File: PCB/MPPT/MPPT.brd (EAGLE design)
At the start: 2 parts, among them IC1 ACS711KEXLT-15AB-T, IC2 ACS711KEXLT-15AB-T

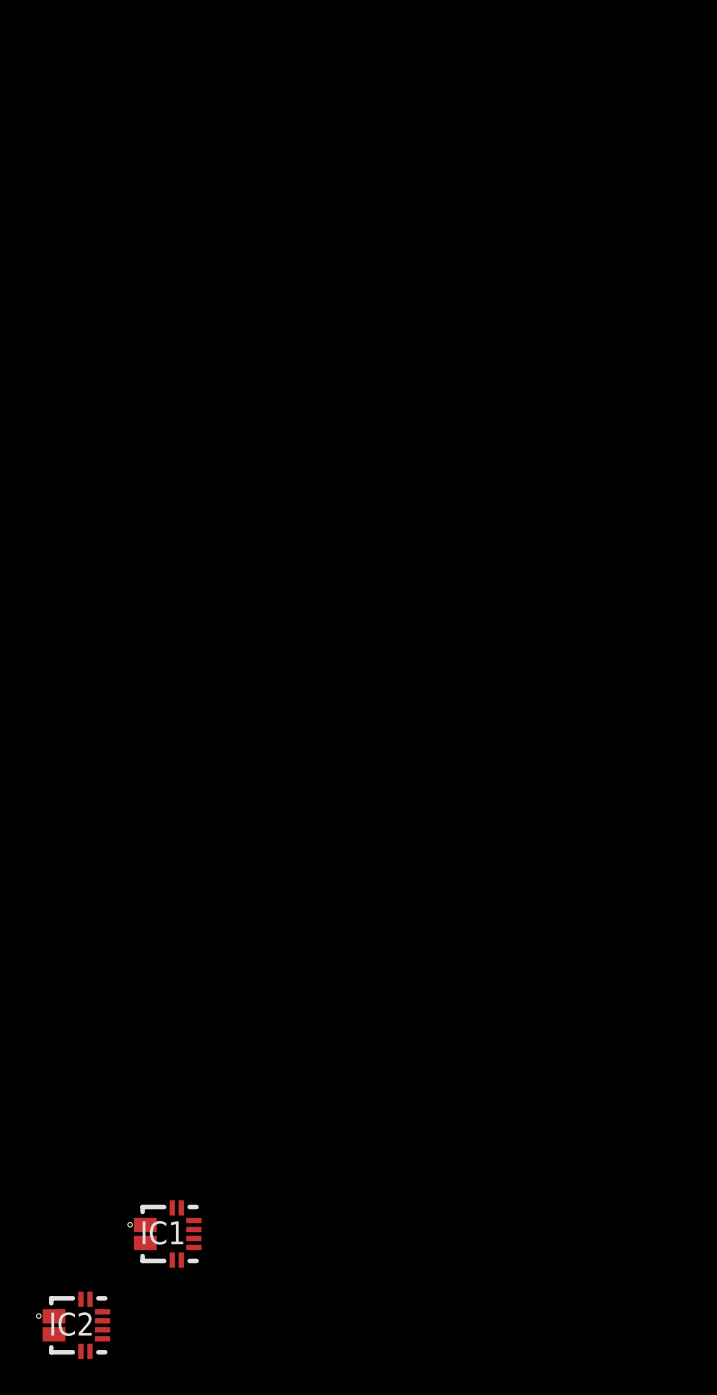
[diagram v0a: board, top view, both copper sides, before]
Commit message: ripup
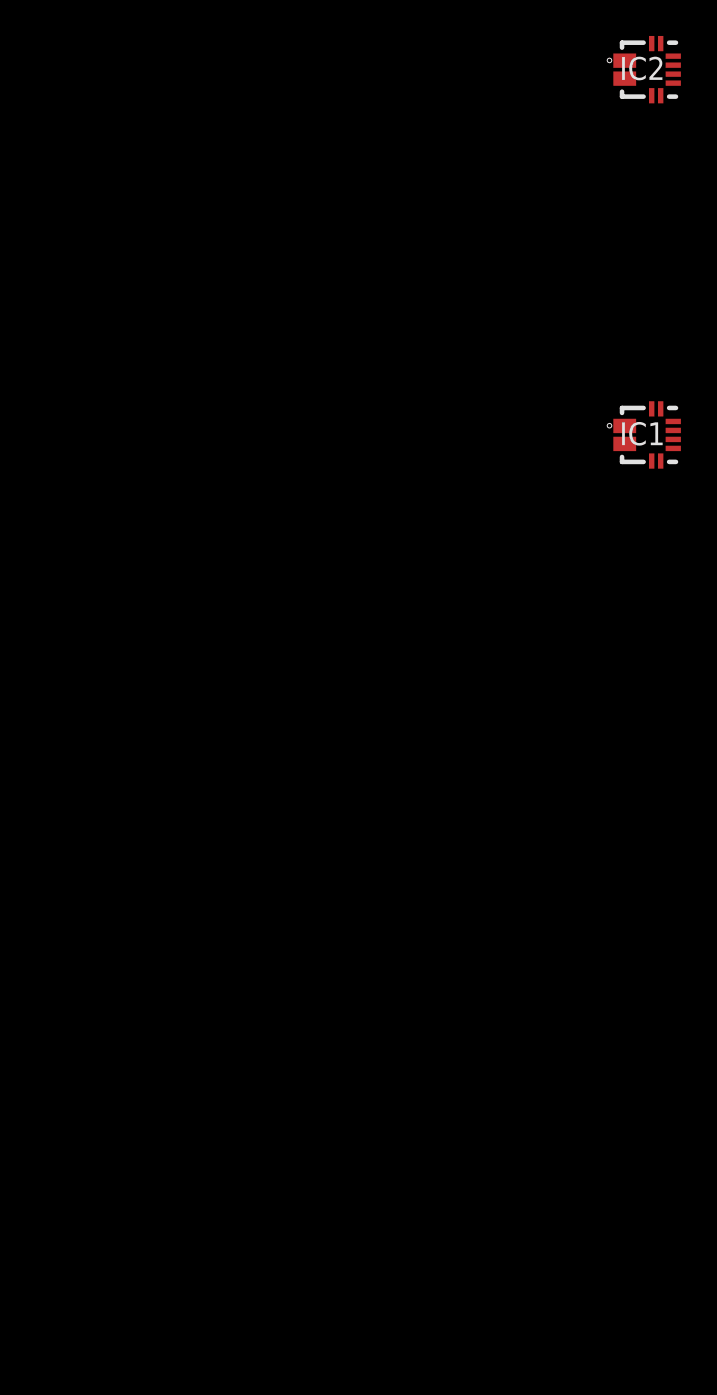
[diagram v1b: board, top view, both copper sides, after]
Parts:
- moved IC2 76.7 mm to (19.1, 49.5)
- moved IC1 51.8 mm to (19.1, 29.2)
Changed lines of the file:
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@@
 </autorouter>
 <elements>
-<element name="IC1" library="SamacSys_Parts" package="EX-PACKAGE" value="ACS711KEXLT-15AB-T" x="-7.62" y="-15.24">
-<attribute name="ARROW_PART_NUMBER" value="ACS711KEXLT-15AB-T" x="-7.62" y="-15.24" size="1.778" layer="27" display="off"/>
-<attribute name="DESCRIPTION" value="Hall Effect Linear Current Sensor with Overcurrent Fault Output for &lt;100 V Isolation Applications" x="-7.62" y="-15.24" size="1.778" layer="27" display="off"/>
-<attribute name="HEIGHT" value="mm" x="-7.62" y="-15.24" size="1.778" layer="27" display="off"/>
-<attribute name="MANUFACTURER_NAME" value="Allegro Microsystems" x="-7.62" y="-15.24" size="1.778" layer="27" display="off"/>
-<attribute name="MANUFACTURER_PART_NUMBER" value="ACS711KEXLT-15AB-T" x="-7.62" y="-15.24" size="1.778" layer="27" display="off"/>
+<element name="IC1" library="SamacSys_Parts" package="EX-PACKAGE" value="ACS711KEXLT-15AB-T" x="19.05" y="29.21">
+<attribute name="ARROW_PART_NUMBER" value="ACS711KEXLT-15AB-T" x="19.05" y="29.21" size="1.778" layer="27" display="off"/>
+<attribute name="DESCRIPTION" value="Hall Effect Linear Current Sensor with Overcurrent Fault Output for &lt;100 V Isolation Applications" x="19.05" y="29.21" size="1.778" layer="27" display="off"/>
+<attribute name="HEIGHT" value="mm" x="19.05" y="29.21" size="1.778" layer="27" display="off"/>
+<attribute name="MANUFACTURER_NAME" value="Allegro Microsystems" x="19.05" y="29.21" size="1.778" layer="27" display="off"/>
+<attribute name="MANUFACTURER_PART_NUMBER" value="ACS711KEXLT-15AB-T" x="19.05" y="29.21" size="1.778" layer="27" display="off"/>
 </element>
-<element name="IC2" library="SamacSys_Parts" package="EX-PACKAGE" value="ACS711KEXLT-15AB-T" x="-12.7" y="-20.32">
-<attribute name="ARROW_PART_NUMBER" value="ACS711KEXLT-15AB-T" x="-12.7" y="-20.32" size="1.778" layer="27" display="off"/>
-<attribute name="DESCRIPTION" value="Hall Effect Linear Current Sensor with Overcurrent Fault Output for &lt;100 V Isolation Applications" x="-12.7" y="-20.32" size="1.778" layer="27" display="off"/>
-<attribute name="HEIGHT" value="mm" x="-12.7" y="-20.32" size="1.778" layer="27" display="off"/>
-<attribute name="MANUFACTURER_NAME" value="Allegro Microsystems" x="-12.7" y="-20.32" size="1.778" layer="27" display="off"/>
-<attribute name="MANUFACTURER_PART_NUMBER" value="ACS711KEXLT-15AB-T" x="-12.7" y="-20.32" size="1.778" layer="27" display="off"/>
+<element name="IC2" library="SamacSys_Parts" package="EX-PACKAGE" value="ACS711KEXLT-15AB-T" x="19.05" y="49.53">
+<attribute name="ARROW_PART_NUMBER" value="ACS711KEXLT-15AB-T" x="19.05" y="49.53" size="1.778" layer="27" display="off"/>
+<attribute name="DESCRIPTION" value="Hall Effect Linear Current Sensor with Overcurrent Fault Output for &lt;100 V Isolation Applications" x="19.05" y="49.53" size="1.778" layer="27" display="off"/>
+<attribute name="HEIGHT" value="mm" x="19.05" y="49.53" size="1.778" layer="27" display="off"/>
+<attribute name="MANUFACTURER_NAME" value="Allegro Microsystems" x="19.05" y="49.53" size="1.778" layer="27" display="off"/>
+<attribute name="MANUFACTURER_PART_NUMBER" value="ACS711KEXLT-15AB-T" x="19.05" y="49.53" size="1.778" layer="27" display="off"/>
 </element>
 </elements>
